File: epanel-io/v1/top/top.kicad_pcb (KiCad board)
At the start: 2 copper layers, 66.5 x 100.8 mm, 132 parts, among them J1 Conn_01x05_Male, J2 Conn_01x05_Female, J3 Conn_01x08_Female, J4 Conn_01x05_Female, J5 Conn_01x08_Female, J6 Conn_01x04_Female, J7 Conn_01x04_Female, U1 Pico, U10 4N35, U11 H11AA1, U12 4N35, U13 H11AA1, U14 4N35, U15 H11AA1, U16 4N35, U17 H11AA1, U18 4N35, U19 H11AA1, U2 H11AA1, U20 4N35, U21 H11AA1, U22 4N35, U3 H11AA1, U4 4N35, U5 H11AA1, U6 4N35, U7 H11AA1, U8 4N35, U9 H11AA1

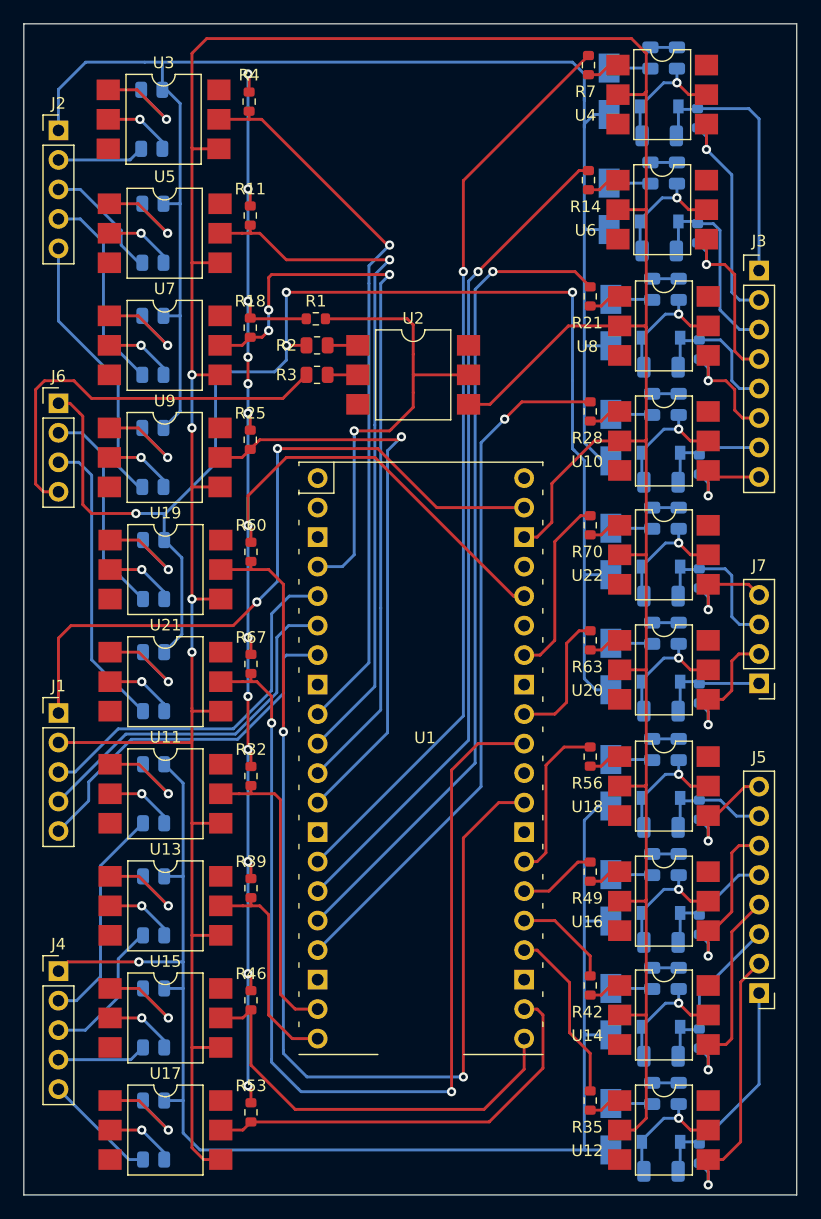
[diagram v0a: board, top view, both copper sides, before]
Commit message: DRC
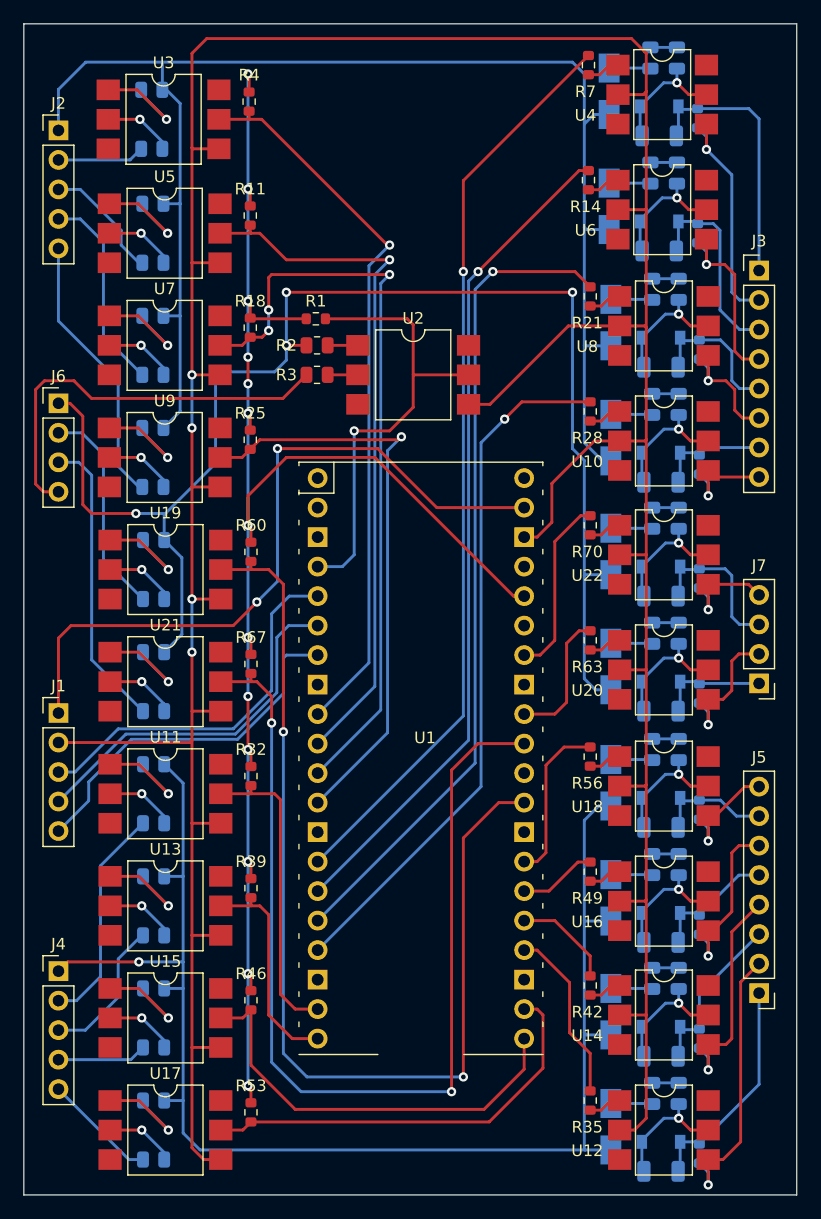
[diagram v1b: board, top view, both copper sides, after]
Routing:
- net /Output 3/GATE: track 11.8 -> 11.1 mm
- net /Output 1/GATE: track 20.8 -> 20.2 mm
- net /Input 1/NEUT: track 128.2 -> 127.7 mm
